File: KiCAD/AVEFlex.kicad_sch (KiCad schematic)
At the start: 35 parts, among them IC1 AVE

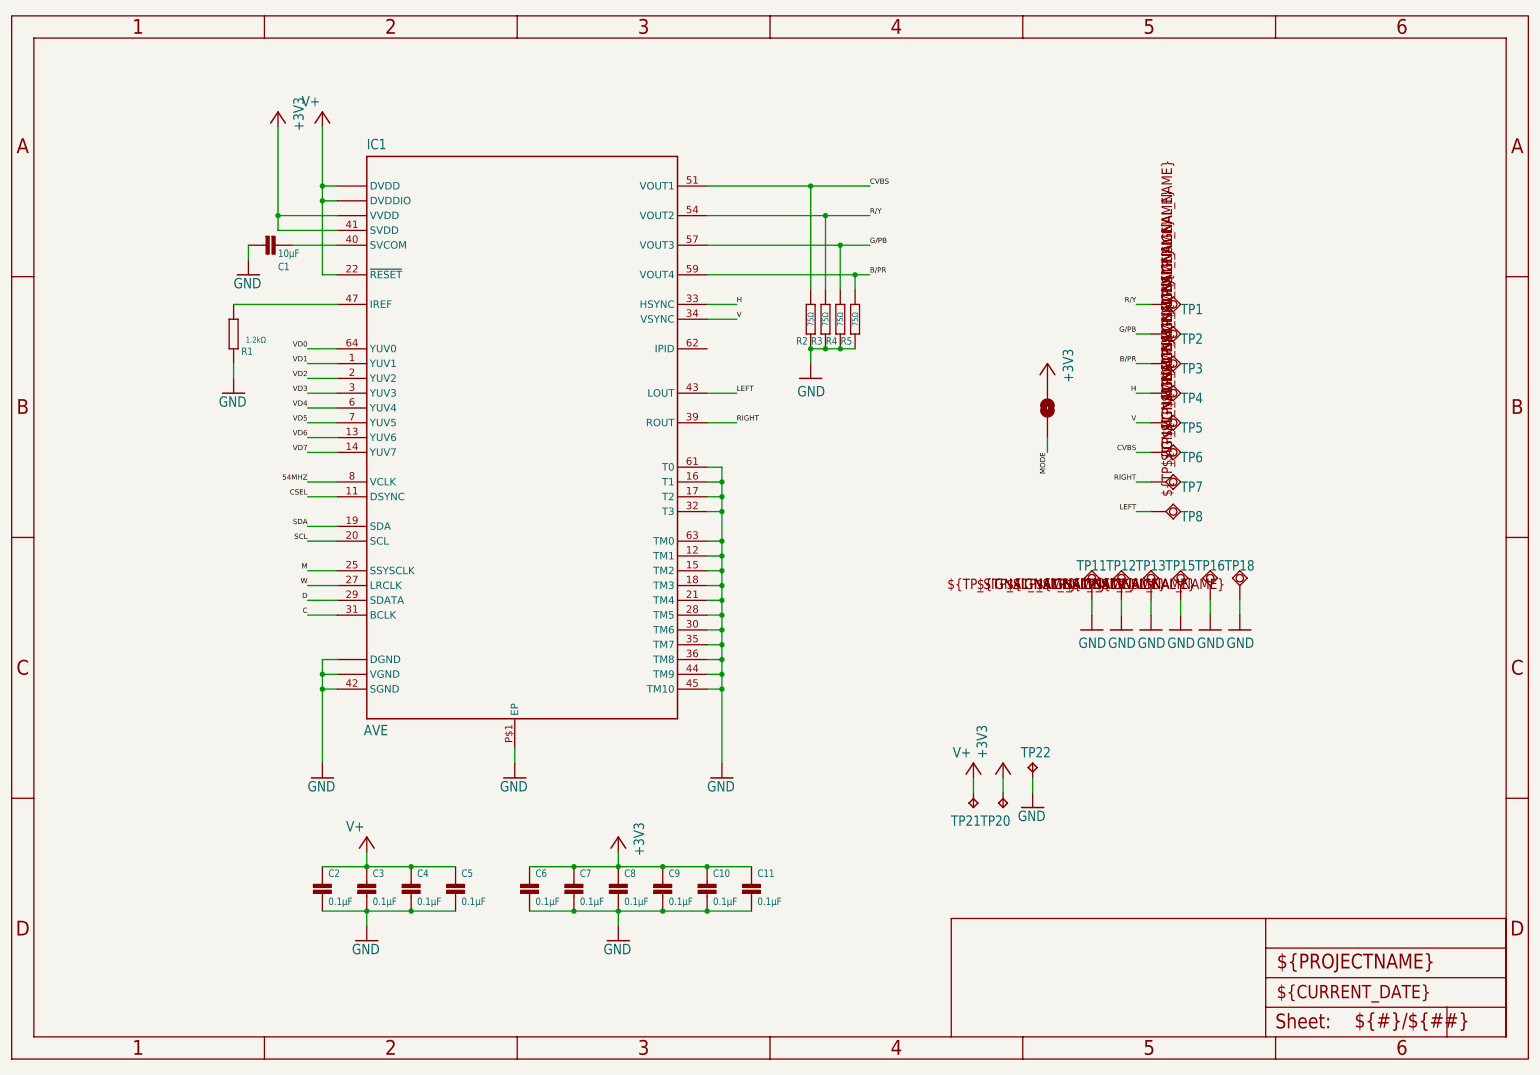
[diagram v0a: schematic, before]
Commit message: Update KiCAD version
- updated KiCAD version
- updated Gerbers
- added new iBOM file
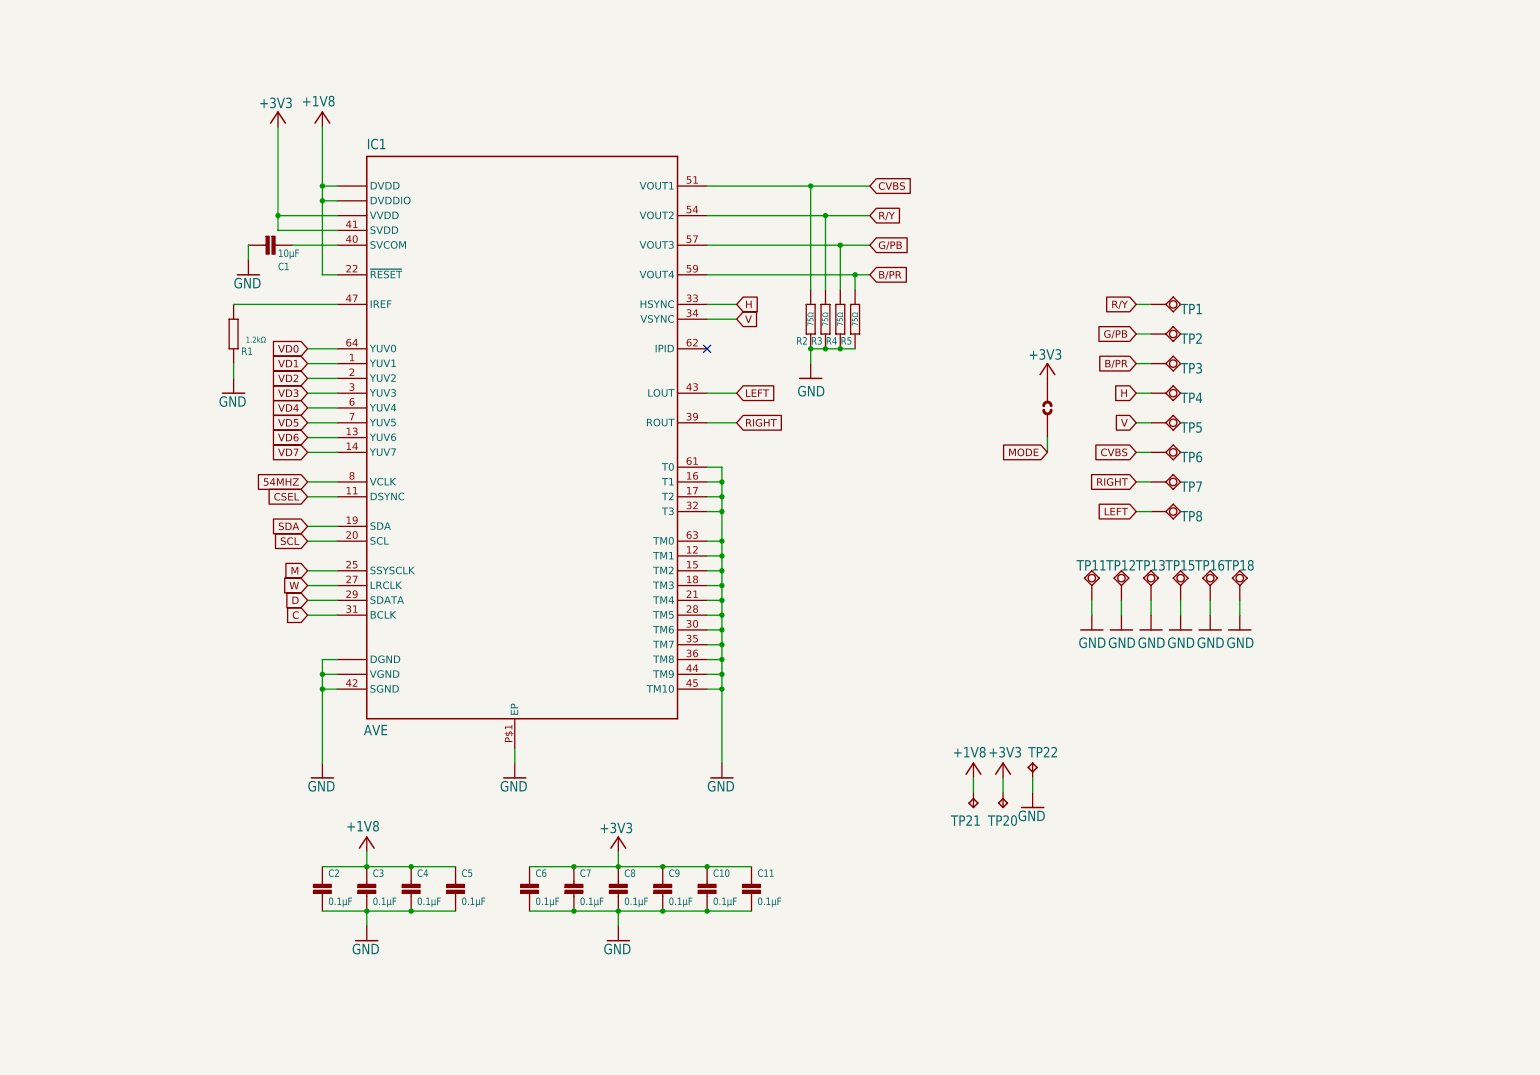
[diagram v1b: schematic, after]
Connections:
- net V+ renamed +1V8
- no-connect marks 0 -> 1
